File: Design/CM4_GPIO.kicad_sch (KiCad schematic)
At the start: 28 parts, among them J1 Conn_01x03, J2 Conn_02x07_Odd_Even, J3 Conn_01x03, J7 Micro_SD_Card_Det, J8 THD-20-R, J9 THD-02-R, U1 TPD4EUSB30, U18 RT9742GGJ5, U2 TPD4EUSB30, U3 MagJack-A70-112-331N126, U5 74LVC1G07SE-7, U9 74LVC1G07SE-7

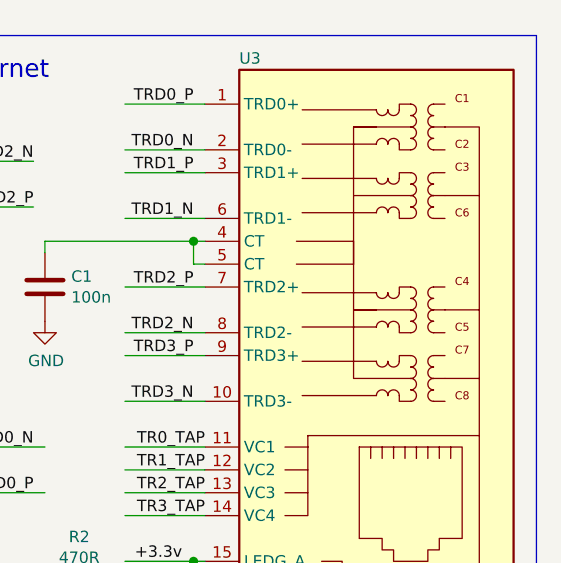
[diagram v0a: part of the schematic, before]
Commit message: project loaded first time
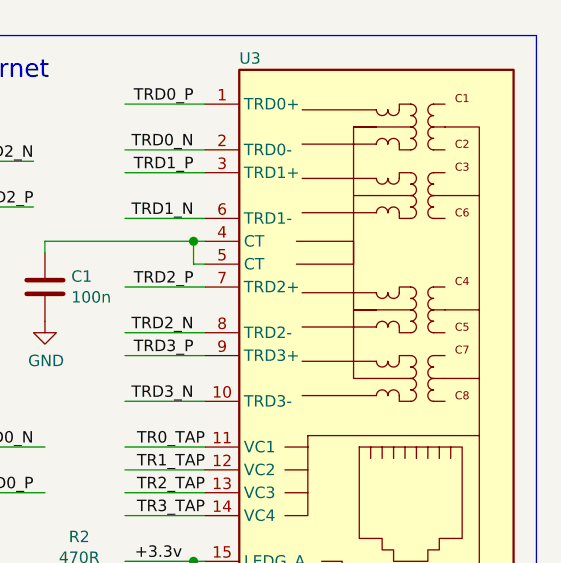
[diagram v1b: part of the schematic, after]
